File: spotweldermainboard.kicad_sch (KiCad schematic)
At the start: 50 parts, among them J1 tft_screen, J2 program, J3 Conn_01x02_Pin, J4 Conn_01x02_Pin, J5 MOT, M1 Motor_DC, M2 Motor_DC, Q1 BC517, Q3 2N7000, Q4 2N7000, U1 CH32V003FxPx, U2 MOC3052M, U3 4N35, U4 BTA40-600B

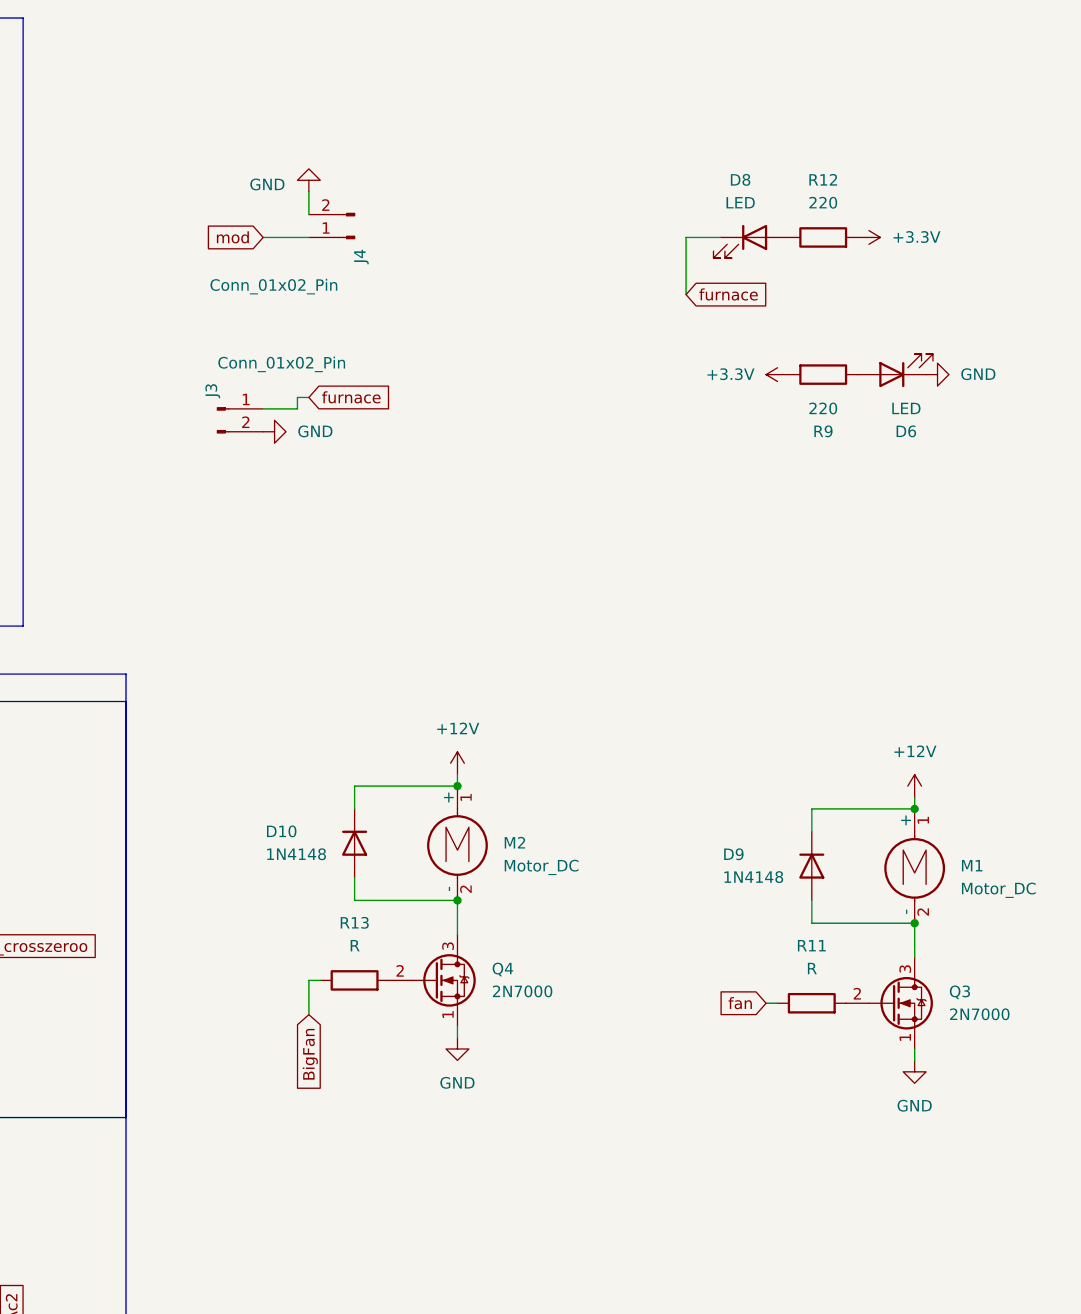
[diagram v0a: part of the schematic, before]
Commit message: block diagrams listos
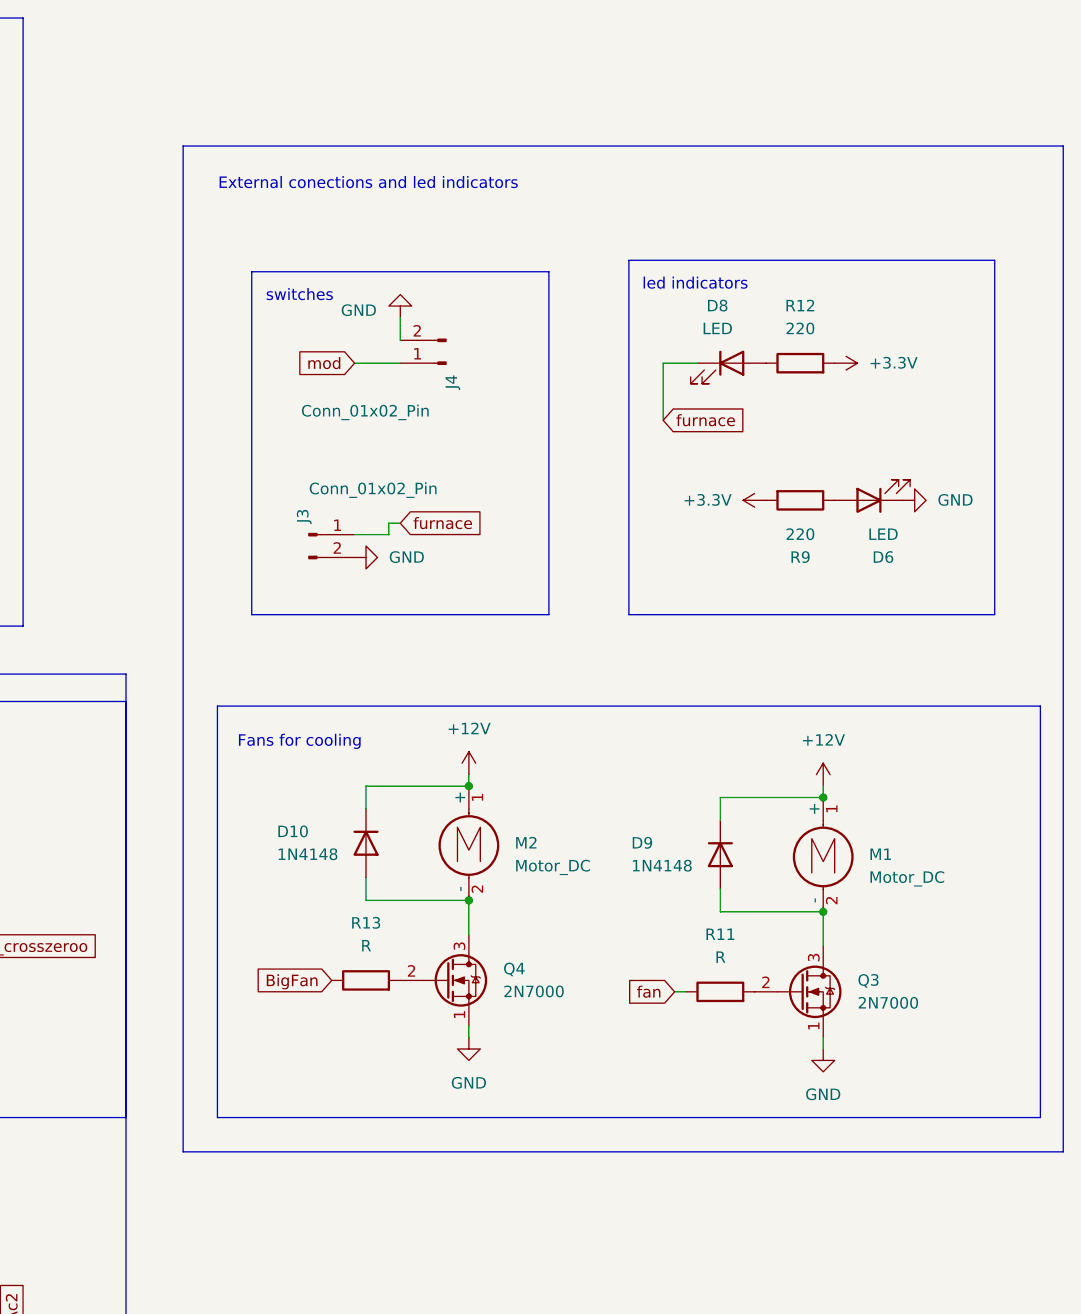
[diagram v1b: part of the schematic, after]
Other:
- note added: "External conections and led indicators"
- note added: "Fans for cooling"
- note added: "led indicators"
- note added: "switches"
- moved on the sheet: D10, D6, D8, D9, J3, J4, M1, M2, Q3, Q4, R11, R12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
